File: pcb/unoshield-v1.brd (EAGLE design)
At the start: 63.5 x 54.6 mm, 11 parts, among them J1 MJ-3536N, J4 ARDUINO_R3_SHIELD, SW3 ON-OFF-ON-360-1013-ND

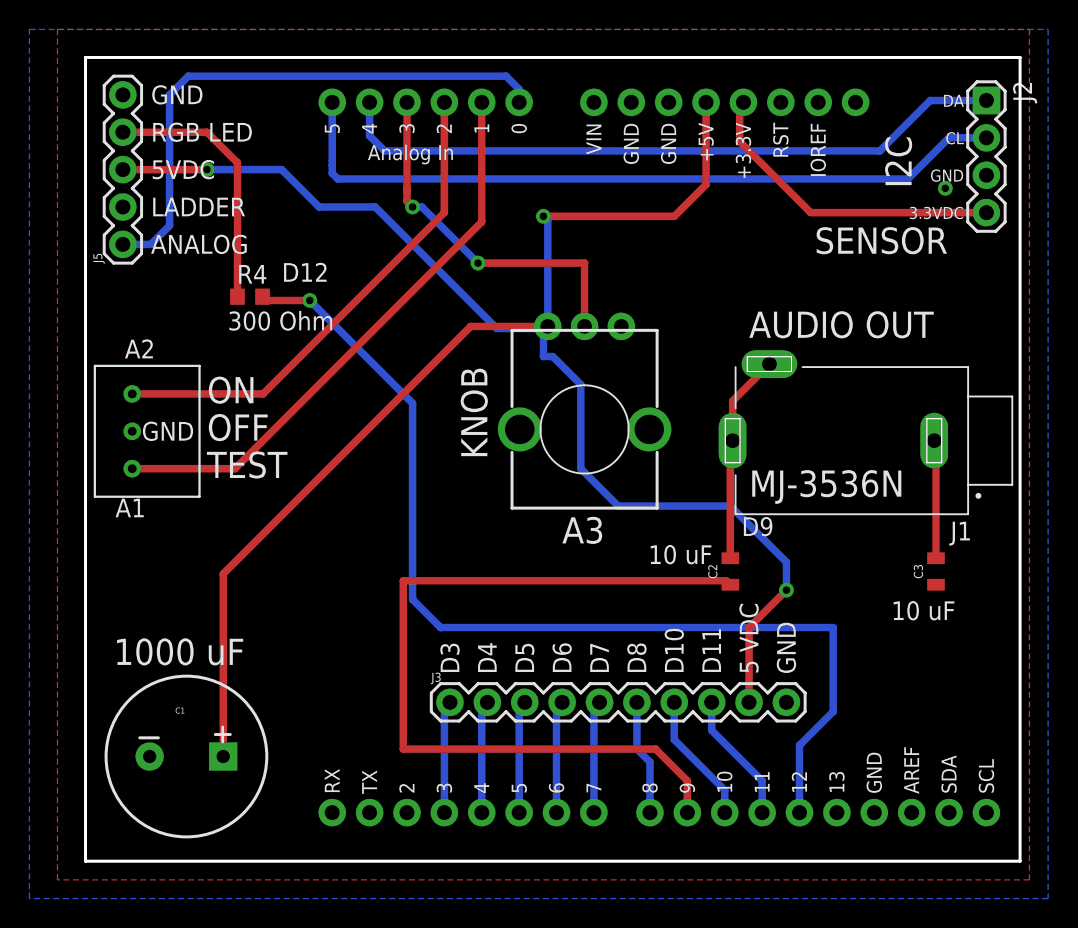
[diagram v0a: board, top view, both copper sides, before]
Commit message: designing circuit boards
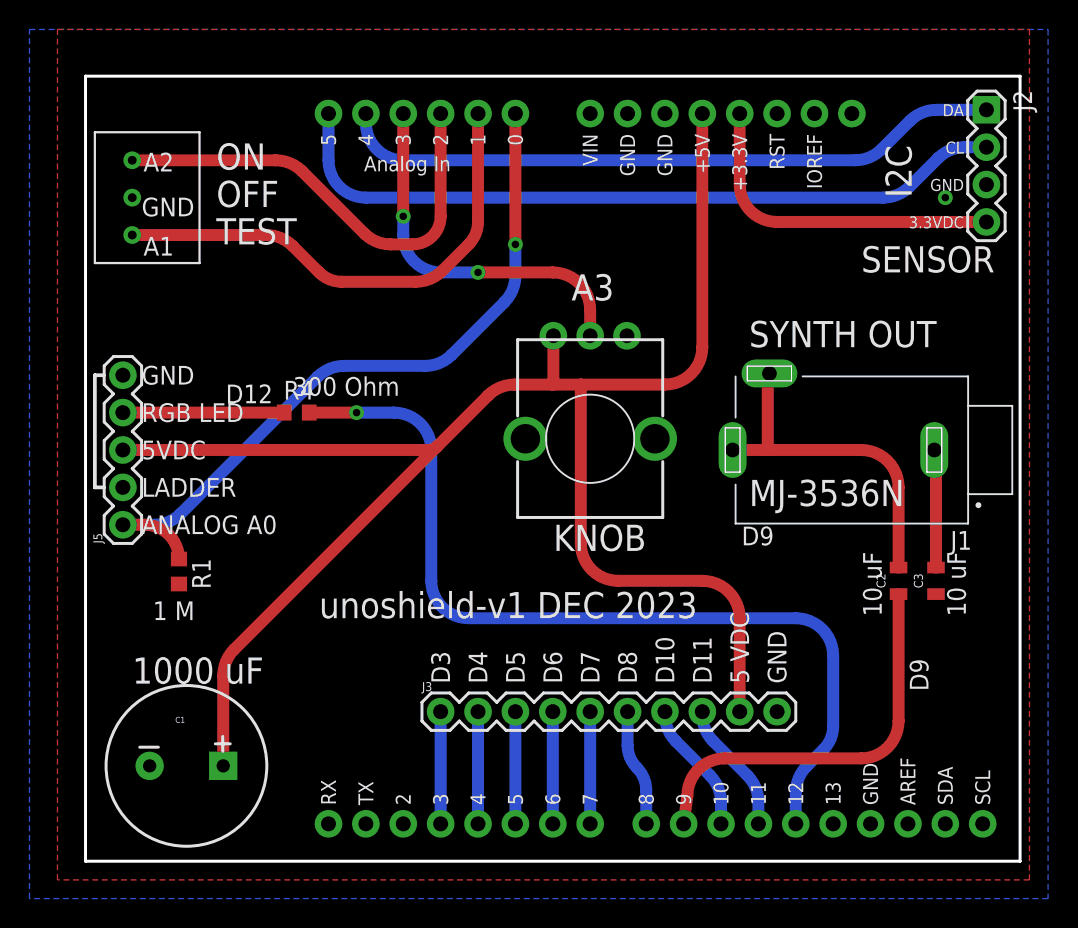
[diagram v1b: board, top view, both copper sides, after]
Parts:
- added R1: 1M, resistor:R0603
- moved J5 19.0 mm to (2.54, 22.9)
- moved SW3 15.9 mm to (3.17, 45.1)
- moved C2 11.4 mm to (55.2, 19.1)
- moved R4 8.49 mm to (14.4, 30.5)
- moved J3 0.90 mm to (24.1, 10.2)
- moved J4 0.80 mm to (71.1, 0.00)
- moved R5 0.74 mm to (34.3, 28.7)
- moved C1 0.63 mm to (6.86, 6.48)
- moved C3 0.63 mm to (57.8, 19.1)
- moved J1 0.63 mm to (52.1, 27.9)
- moved J2 0.63 mm to (61.2, 51.1)
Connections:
- net ANALOG: now also R1.1
- net GND: now also R1.2
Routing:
- net N$16: track 56.1 -> 27.0 mm
- net 5V: track 138.3 -> 118.9 mm, vias 3 -> 0
- net ANALOG: track 38.1 -> 49.4 mm, vias 0 -> 1
- net N$1: track 69.4 -> 60.1 mm
- net N$15: track 14.3 -> 23.0 mm
- net N$17: track 17.7 -> 11.0 mm
- net BUTTON: track 38.8 -> 33.8 mm
- net N$12: track 33.8 -> 30.8 mm
- net VCC: track 21.5 -> 22.6 mm
- net DA: track 46.0 -> 45.0 mm
- net CL: track 50.6 -> 50.0 mm
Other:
- board size 63.5 x 54.6 mm -> 63.5 x 53.3 mm
- board text added: "1 M"
- board text added: "ANALOG A0"
- board text added: "SYNTH OUT"
- board text added: "unoshield-v1 DEC 2023"
- board text removed: "ANALOG"
- board text removed: "AUDIO OUT"
